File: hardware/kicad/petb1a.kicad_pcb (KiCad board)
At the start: 2 copper layers, 22.9 x 58.4 mm, 31 parts, among them J1 TYPEC-304-ACP16, J2 DNP, J3 DNP, SW1 TD-1183SA-1.5H-250, SW2 TD-1183SA-1.5H-250, U1 USBLC6-2P6, U2 ESP32-S3-WROOM-1, U3 XC6220B331MR-G

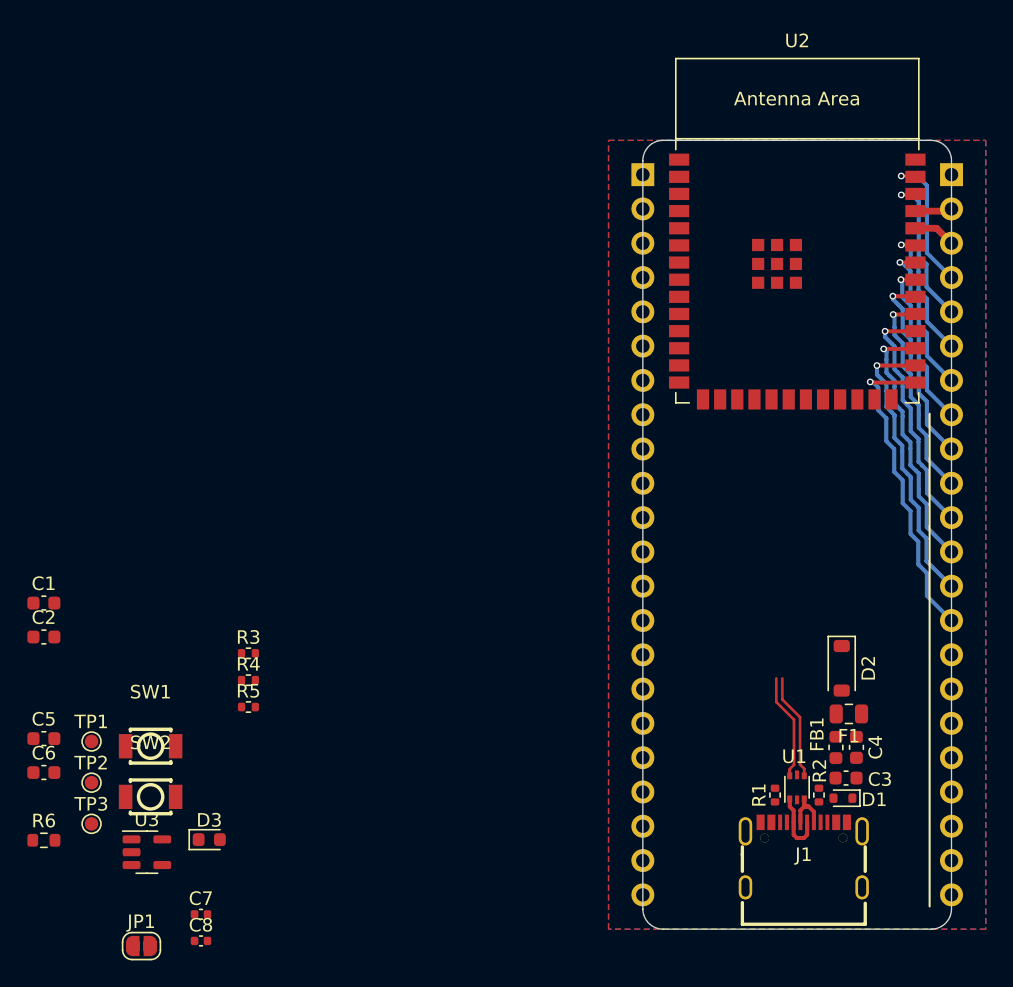
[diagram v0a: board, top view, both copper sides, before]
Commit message: update pcb layout
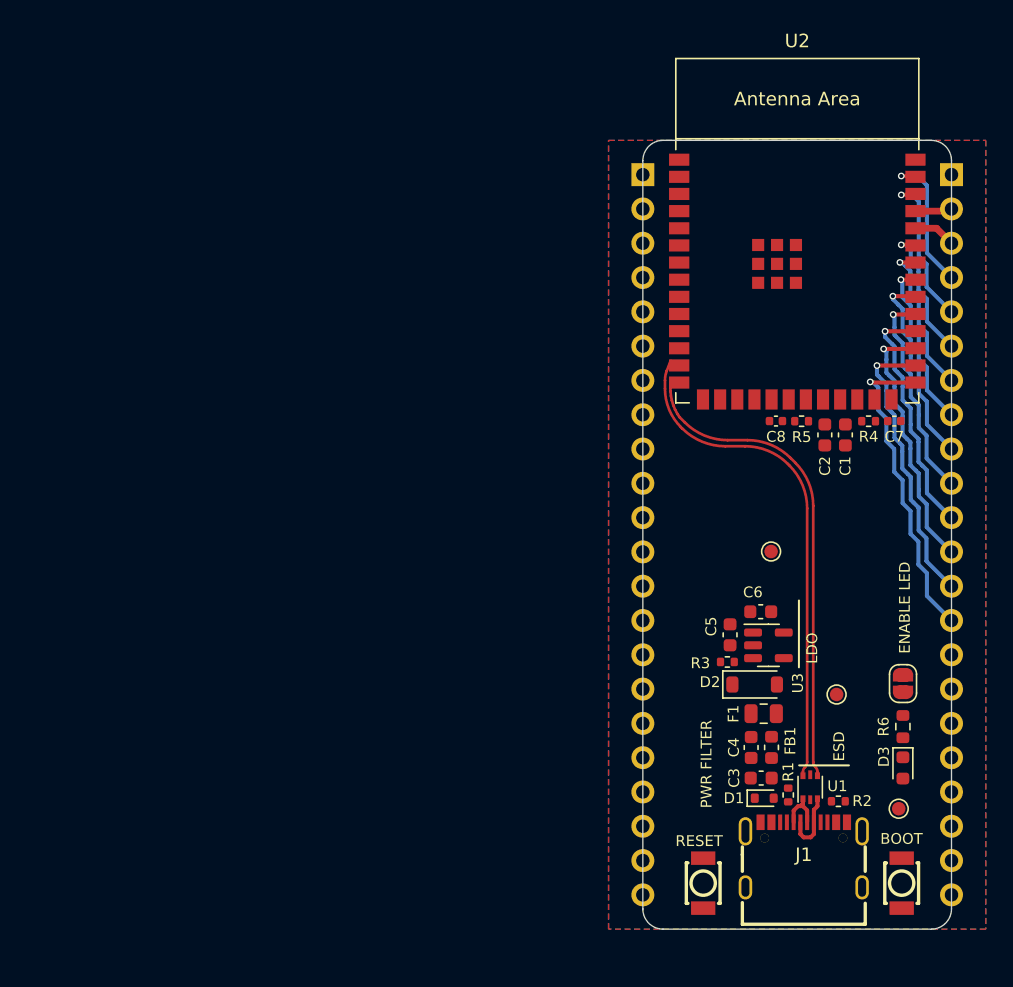
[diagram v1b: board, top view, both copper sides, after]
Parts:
- moved R6 64.2 mm to (156.4, 104.4), turned to 90 degrees
- moved C7 63.0 mm to (155.8, 81.8)
- moved C1 60.7 mm to (152.2, 82.8), turned to -90 degrees
- moved TP1 60.0 mm to (156.1, 110.5)
- moved C2 59.7 mm to (150.6, 82.8), turned to -90 degrees
- moved JP1 59.7 mm to (156.4, 101.2), turned to -90 degrees
- moved C8 57.4 mm to (147.0, 81.8), turned to 180 degrees
- moved SW1 56.5 mm to (156.3, 116.0), turned to 90 degrees
- moved TP2 55.6 mm to (151.5, 102.0)
- moved C6 54.4 mm to (145.9, 95.9), turned to 180 degrees
- moved TP3 54.2 mm to (146.7, 91.4)
- moved D3 51.6 mm to (156.4, 107.4), turned to -90 degrees
- moved C5 51.4 mm to (143.6, 97.6), turned to 90 degrees
- moved R4 49.8 mm to (153.9, 81.8)
- moved U3 48.5 mm to (146.5, 98.4)
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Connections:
- D3 pad 2: Net-(D3-A) -> +3V3
- JP1 pad 2: Net-(D3-K) -> Net-(JP1-B)
- R6 pad 1: +3V3 -> Net-(D3-K)
- R6 pad 2: Net-(D3-A) -> Net-(JP1-B)
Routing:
- net /D_OUT-: track 7.88 -> 37.5 mm
- net /D_OUT+: track 7.88 -> 36.5 mm
- net /D_IN-: track 4.91 -> 3.83 mm
- net /D_IN+: track 3.90 -> 4.81 mm
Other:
- board text added: "BOOT"
- board text added: "ENABLE LED"
- board text added: "ESD"
- board text added: "LDO"
- board text added: "PWR FILTER"
- board text added: "RESET"
